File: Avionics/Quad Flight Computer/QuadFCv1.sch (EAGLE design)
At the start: 126 parts, among them J2 1050270001, Q1 DMP2035U, Q2 DMP2035U, Q3 DMP2035U, SW1 PTS635VL31-VERT, U1 TM4C123GH6PZ, U10 LTC4412, U11 AP7215-33YG-13, U2 74LVC4245APW, U3 ATMEGA32U2-MU, U4 MCP6L91T-E/OT, U5 INVESENSE_MPU-6000, U6 HMC5883LSMD, U7 MS5611-01BA, U8 74AUP1G19GW, U9 S25FL127S, X1 HWB, Y1 32.768KHZ, Y2 AWSCR-20.00CW-T, Y3 PRQC16.00SR5010X000

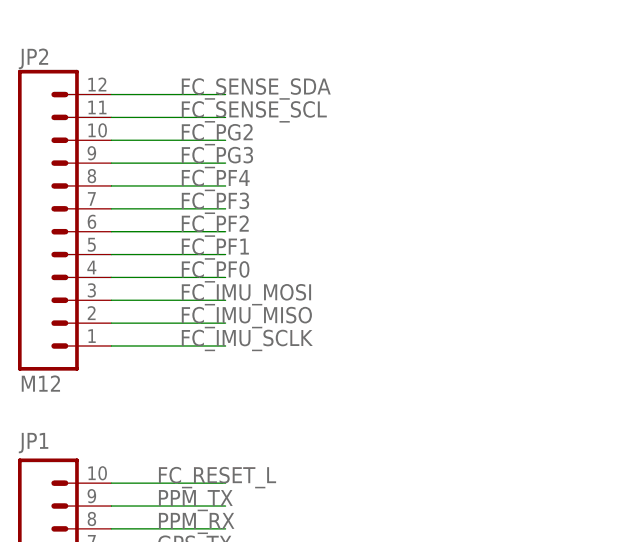
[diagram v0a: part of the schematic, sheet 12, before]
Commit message: More routing
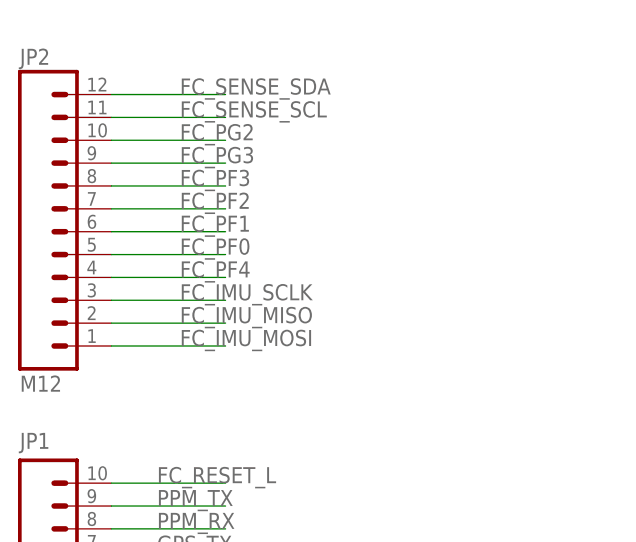
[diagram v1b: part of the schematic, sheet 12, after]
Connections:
- net FC_IMU_MOSI: now also JP2.1; no longer JP2.3
- net FC_IMU_SCLK: now also JP2.3; no longer JP2.1
- net FC_PF0: now also JP2.5; no longer JP2.4
- net FC_PF1: now also JP2.6; no longer JP2.5
- net FC_PF2: now also JP2.7; no longer JP2.6
- net FC_PF3: now also JP2.8; no longer JP2.7
- net FC_PF4: now also JP2.4; no longer JP2.8
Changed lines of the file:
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@@
 <net name="FC_IMU_SCLK" class="0">
 <segment>
-<pinref part="JP2" gate="G$1" pin="1"/>
-<wire x1="-35.56" y1="7.62" x2="-22.86" y2="7.62" width="0.1524" layer="91"/>
-<label x="-27.94" y="7.62" size="1.778" layer="95"/>
+<pinref part="JP2" gate="G$1" pin="3"/>
+<wire x1="-35.56" y1="12.7" x2="-22.86" y2="12.7" width="0.1524" layer="91"/>
+<label x="-27.94" y="12.7" size="1.778" layer="95"/>
 </segment>
 </net>
@@
 </segment>
 </net>
-<net name="FC_IMU_MOSI" class="0">
-<segment>
-<pinref part="JP2" gate="G$1" pin="3"/>
-<wire x1="-35.56" y1="12.7" x2="-22.86" y2="12.7" width="0.1524" layer="91"/>
-<label x="-27.94" y="12.7" size="1.778" layer="95"/>
-</segment>
-</net>
 <net name="FC_SENSE_SCL" class="0">
 <segment>
@@
 <net name="FC_PF1" class="0">
 <segment>
+<wire x1="-35.56" y1="20.32" x2="-22.86" y2="20.32" width="0.1524" layer="91"/>
+<label x="-27.94" y="20.32" size="1.778" layer="95"/>
+<pinref part="JP2" gate="G$1" pin="6"/>
+</segment>
+</net>
+<net name="FC_PF0" class="0">
+<segment>
+<wire x1="-22.86" y1="17.78" x2="-35.56" y2="17.78" width="0.1524" layer="91"/>
+<label x="-27.94" y="17.78" size="1.778" layer="95"/>
 <pinref part="JP2" gate="G$1" pin="5"/>
-<wire x1="-35.56" y1="17.78" x2="-22.86" y2="17.78" width="0.1524" layer="91"/>
-<label x="-27.94" y="17.78" size="1.778" layer="95"/>
-</segment>
-</net>
-<net name="FC_PF0" class="0">
-<segment>
-<pinref part="JP2" gate="G$1" pin="4"/>
-<wire x1="-22.86" y1="15.24" x2="-35.56" y2="15.24" width="0.1524" layer="91"/>
-<label x="-27.94" y="15.24" size="1.778" layer="95"/>
 </segment>
 </net>
@@
 <net name="FC_PF2" class="0">
 <segment>
-<pinref part="JP2" gate="G$1" pin="6"/>
-<wire x1="-22.86" y1="20.32" x2="-35.56" y2="20.32" width="0.1524" layer="91"/>
-<label x="-27.94" y="20.32" size="1.778" layer="95"/>
+<wire x1="-22.86" y1="22.86" x2="-35.56" y2="22.86" width="0.1524" layer="91"/>
+<label x="-27.94" y="22.86" size="1.778" layer="95"/>
+<pinref part="JP2" gate="G$1" pin="7"/>
 </segment>
 </net>
 <net name="FC_PF3" class="0">
 <segment>
-<pinref part="JP2" gate="G$1" pin="7"/>
-<wire x1="-35.56" y1="22.86" x2="-22.86" y2="22.86" width="0.1524" layer="91"/>
-<label x="-27.94" y="22.86" size="1.778" layer="95"/>
+<wire x1="-35.56" y1="25.4" x2="-22.86" y2="25.4" width="0.1524" layer="91"/>
+<label x="-27.94" y="25.4" size="1.778" layer="95"/>
+<pinref part="JP2" gate="G$1" pin="8"/>
 </segment>
 </net>
@@
 <net name="FC_PF4" class="0">
 <segment>
-<pinref part="JP2" gate="G$1" pin="8"/>
-<wire x1="-35.56" y1="25.4" x2="-22.86" y2="25.4" width="0.1524" layer="91"/>
-<label x="-27.94" y="25.4" size="1.778" layer="95"/>
+<pinref part="JP2" gate="G$1" pin="4"/>
+<wire x1="-22.86" y1="15.24" x2="-35.56" y2="15.24" width="0.1524" layer="91"/>
+<label x="-27.94" y="15.24" size="1.778" layer="95"/>
 </segment>
 </net>
@@
 </segment>
 </net>
+<net name="FC_IMU_MOSI" class="0">
+<segment>
+<pinref part="JP2" gate="G$1" pin="1"/>
+<wire x1="-35.56" y1="7.62" x2="-22.86" y2="7.62" width="0.1524" layer="91"/>
+<label x="-27.94" y="7.62" size="1.778" layer="95"/>
+</segment>
+</net>
